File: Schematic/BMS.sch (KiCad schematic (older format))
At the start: 0 parts

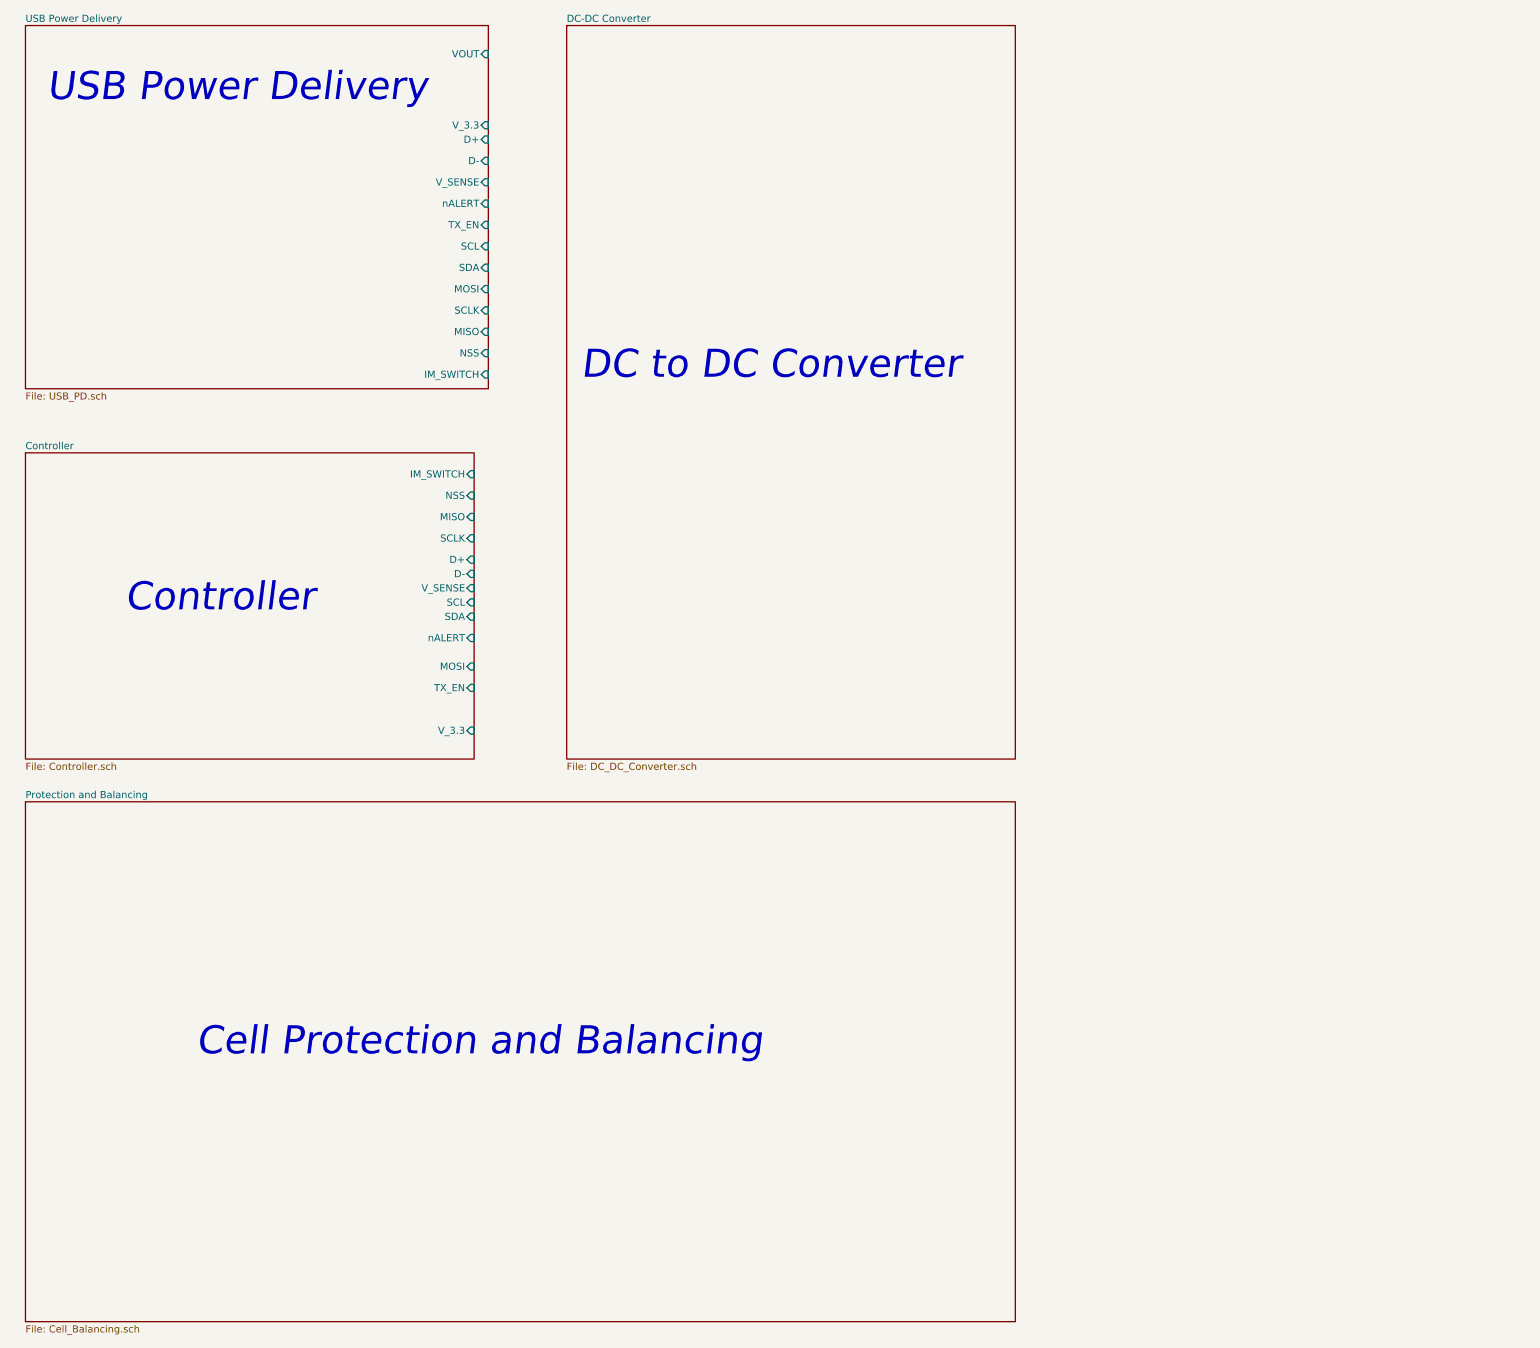
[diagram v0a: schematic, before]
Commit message: Add files via upload
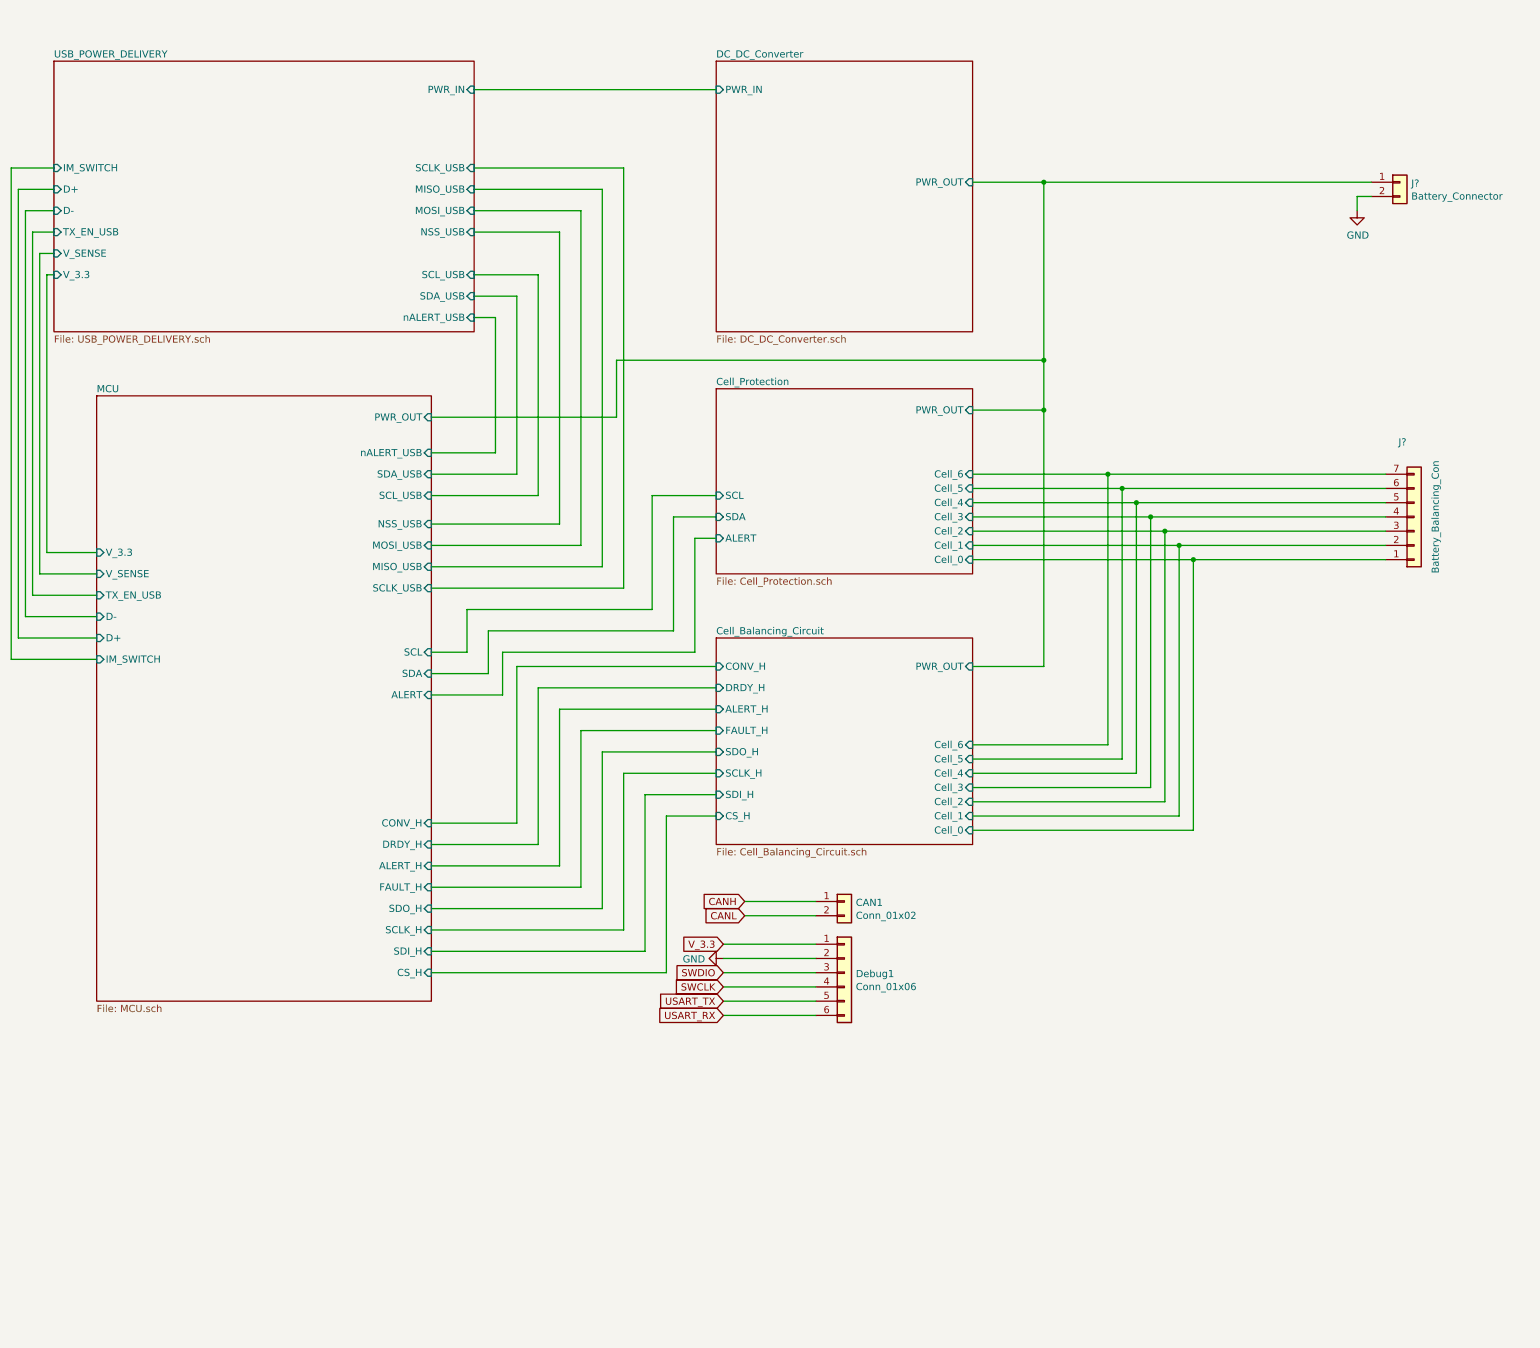
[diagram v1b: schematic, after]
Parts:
- added CAN1: Conn_01x02, symbol Connector_Generic:Conn_01x02
- added Debug1: Conn_01x06, symbol Connector_Generic:Conn_01x06
- added J?: Battery_Connector, symbol Connector_Generic:Conn_01x02
- added J?: Battery_Balancing_Con, symbol Connector_Generic:Conn_01x07
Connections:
- new net CANH: CAN1.1 (Pin_1)
- new net CANL: CAN1.2 (Pin_2)
- new net Cell_Balancing_Circuit/Cell_0: J?.1 (Pin_1)
- new net Cell_Balancing_Circuit/Cell_1: J?.2 (Pin_2)
- new net Cell_Balancing_Circuit/Cell_2: J?.3 (Pin_3)
- new net Cell_Balancing_Circuit/Cell_3: J?.4 (Pin_4)
- new net Cell_Balancing_Circuit/Cell_4: J?.5 (Pin_5)
- new net Cell_Balancing_Circuit/Cell_5: J?.6 (Pin_6)
- new net Cell_Balancing_Circuit/Cell_6: J?.7 (Pin_7)
- new net Cell_Balancing_Circuit/PWR_OUT: J?.1 (Pin_1)
- new net GND: Debug1.2 (Pin_2), J?.2 (Pin_2)
- new net SWCLK: Debug1.4 (Pin_4)
- new net SWDIO: Debug1.3 (Pin_3)
- new net USART_RX: Debug1.6 (Pin_6)
- new net USART_TX: Debug1.5 (Pin_5)
- new net V_3.3: Debug1.1 (Pin_1)
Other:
- note removed: "Cell Protection and Balancing"
- note removed: "Controller\n\n"
- note removed: "DC to DC Converter\n"
- note removed: "USB Power Delivery"
